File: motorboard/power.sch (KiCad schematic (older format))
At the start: 18 parts, among them Q3 PMV20ENR, U13 TPS2412PW, U4 TPS63070

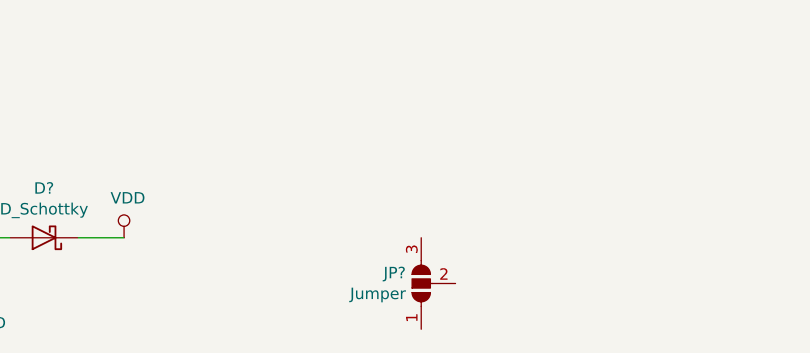
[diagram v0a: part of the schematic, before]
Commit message: neater
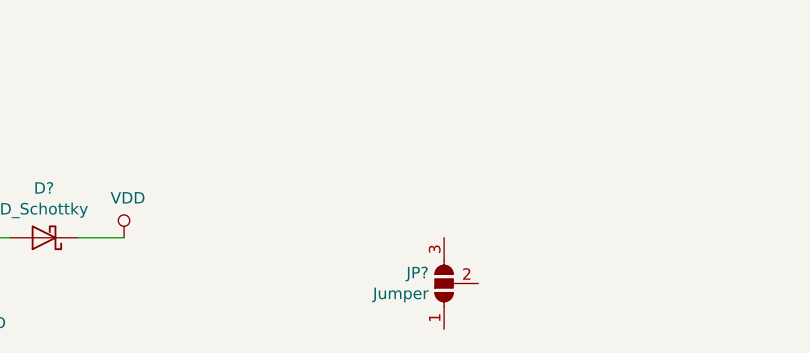
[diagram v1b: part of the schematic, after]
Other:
- moved on the sheet: JP?
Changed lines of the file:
@@
 L Jumper:SolderJumper_3_Open JP?
 U 1 1 5E8D85AC
-P 3850 7000
-F 0 "JP?" V 3896 7067 50  0000 L CNN
-F 1 "Jumper" V 3805 7067 50  0000 L CNN
-F 2 "" H 3850 7000 50  0001 C CNN
-F 3 "~" H 3850 7000 50  0001 C CNN
-	1    3850 7000
+P 3950 7000
+F 0 "JP?" V 3996 7067 50  0000 L CNN
+F 1 "Jumper" V 3905 7067 50  0000 L CNN
+F 2 "" H 3950 7000 50  0001 C CNN
+F 3 "~" H 3950 7000 50  0001 C CNN
+	1    3950 7000
 	0    -1   -1   0
 $EndComp
